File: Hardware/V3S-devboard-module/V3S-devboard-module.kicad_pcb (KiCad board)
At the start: 4 copper layers, 31.9 x 52.9 mm, 84 parts, among them J101 Conn_01x02, J201 Micro_SD_Card_Det1, J301 AS0BC21-S30BE-7H, SW201 SW_MEC_5E, U101 EA3036C, U102 XC6206PxxxMR, U201 V3S, U202 W25Q128JVS, Y201 Crystal_Small, Y202 Crystal_GND24_Small

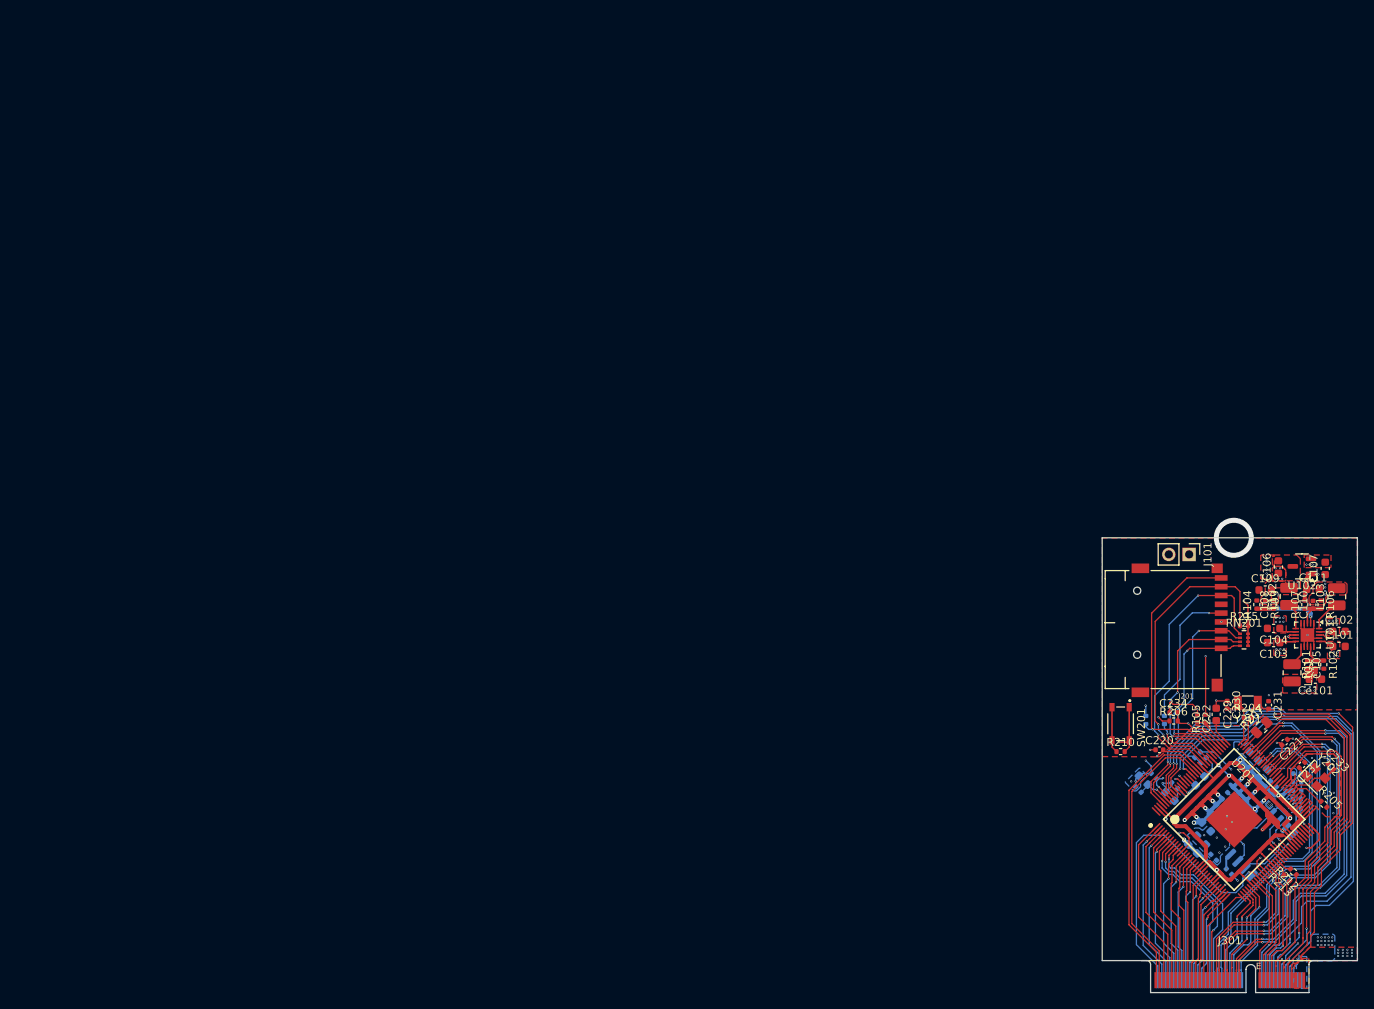
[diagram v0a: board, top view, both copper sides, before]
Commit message: started working on exp board
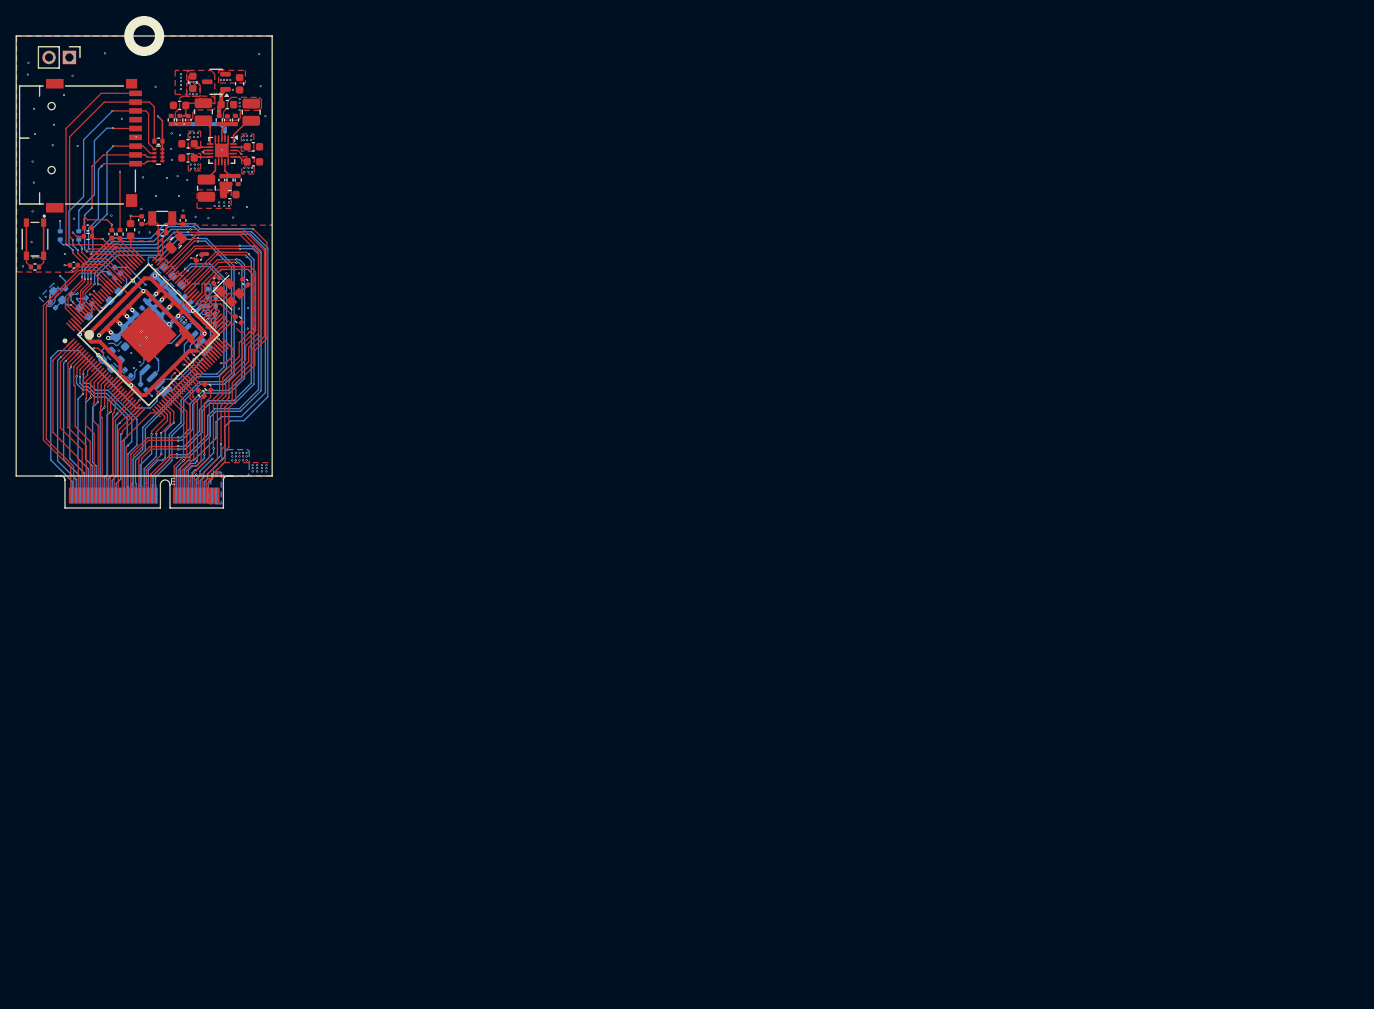
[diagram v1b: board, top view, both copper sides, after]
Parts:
- moved J101 153.1 mm to (6.64, 2.68)
- moved C103 148.6 mm to (21.5, 15.2)
- moved C104 148.6 mm to (21.5, 13.5)
- moved C105 148.6 mm to (25.7, 18.0)
- moved C108 148.6 mm to (21.5, 10.5)
- moved C109 148.6 mm to (20.4, 8.68)
- moved C111 148.6 mm to (26.4, 8.57)
- moved C202 148.6 mm to (24.4, 34.8)
- moved C203 148.6 mm to (19.0, 30.5)
- moved C204 148.6 mm to (20.1, 31.6)
- moved C207 148.6 mm to (20.8, 32.9)
- moved C208 148.6 mm to (18.4, 36.8)
- moved C210 148.6 mm to (16.8, 34.4)
- moved C211 148.6 mm to (16.1, 33.7)
- moved C213 148.6 mm to (12.5, 41.0)
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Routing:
- net 5V: track 41.3 -> 45.0 mm
- net 1V2: track 179.8 -> 178.9 mm
- net GND: vias 54 -> 95
- net (no net): vias 1 -> 0
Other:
- board size 31.9 x 52.9 mm -> 32 x 55 mm
